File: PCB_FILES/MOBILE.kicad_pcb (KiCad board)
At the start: 2 copper layers, 88.6 x 52.6 mm, 33 parts, among them J1 Conn_01x05_Pin, Q1 MMBT3904_C181119, U1 HT7833, U2 ESP32-WROOM-32E-N8R2

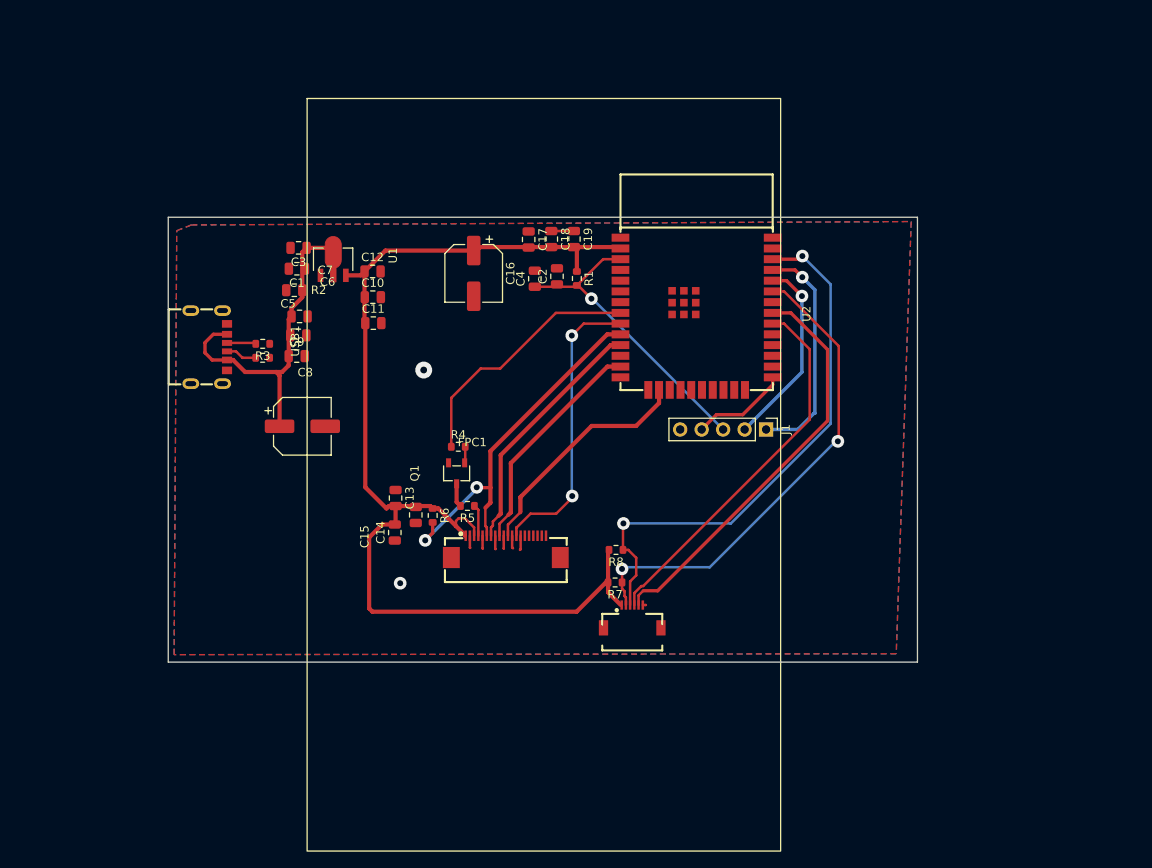
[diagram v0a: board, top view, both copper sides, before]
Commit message: 3rd commit
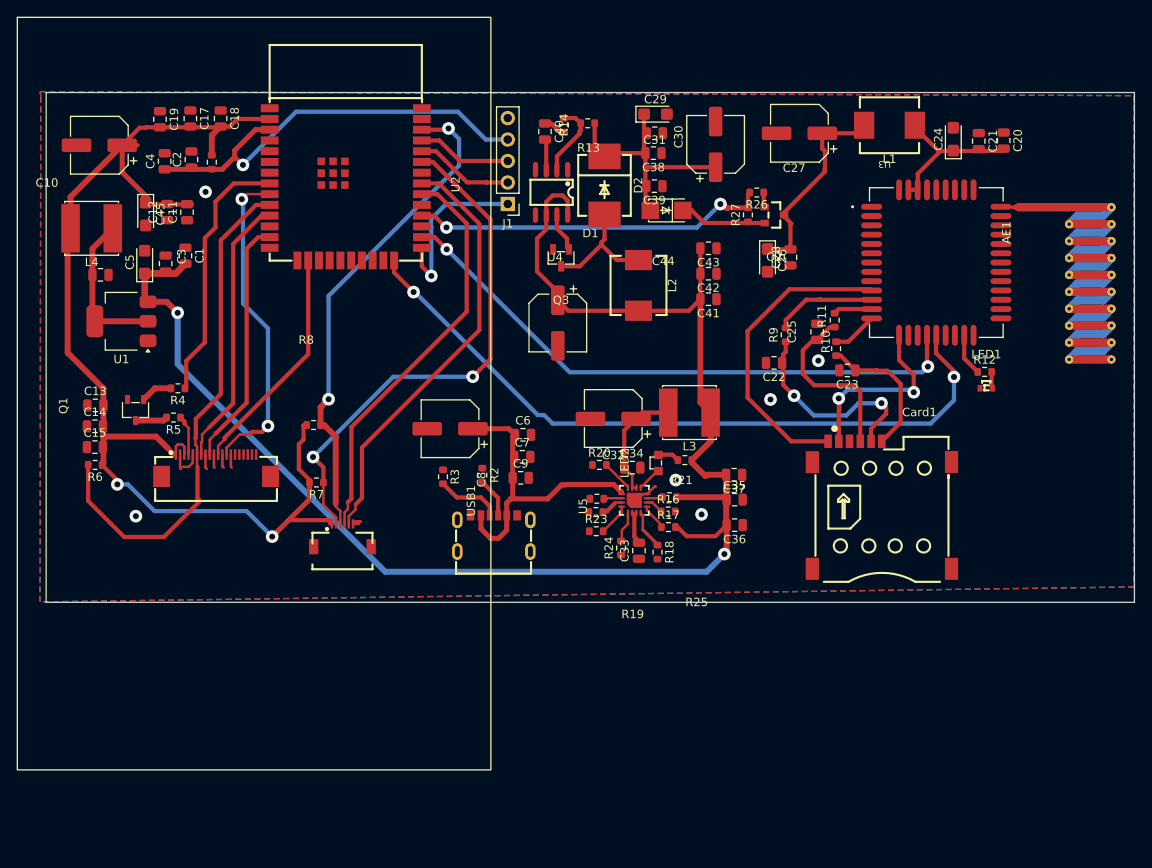
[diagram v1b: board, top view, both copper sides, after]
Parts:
- added AE1: Antenna, RF_Antenna:Texas_SWRA416_868MHz_915MHz, F.Cu at (159.2, 127.2)
- added C20: 100nF, Capacitor_SMD:C_0805_2012Metric, F.Cu at (152.3, 110.3)
- added C21: 33pF, Capacitor_SMD:C_0805_2012Metric, F.Cu at (149.3, 110.4)
- added C22: 33pF, Capacitor_SMD:C_0805_2012Metric, F.Cu at (125.1, 136.6)
- added C23: 33pF, Capacitor_SMD:C_0805_2012Metric, F.Cu at (133.8, 137.5)
- added C24: TAN 100uF, Capacitor_Tantalum_SMD:CP_EIA-3216-18_Kemet-A, F.Cu at (146.3, 110.2)
- added C25: 33pF, Capacitor_SMD:C_0805_2012Metric, F.Cu at (130.2, 133.0)
- added C26: TAN 100uF, Capacitor_Tantalum_SMD:CP_EIA-3216-18_Kemet-A, F.Cu at (124.4, 124.5)
- added C27: 470uF, Capacitor_SMD:CP_Elec_6.3x7.7, F.Cu at (128.1, 109.5)
- added C28: 22uF, Capacitor_SMD:C_0805_2012Metric, F.Cu at (127.1, 124.2)
- added C29: TAN 100uF, Capacitor_Tantalum_SMD:CP_EIA-3216-18_Kemet-A, F.Cu at (111.1, 107.2)
- added C30: 470uF, Capacitor_SMD:CP_Elec_6.3x7.7, F.Cu at (118.2, 110.8)
- added C31: 33pF, Capacitor_SMD:C_0805_2012Metric, F.Cu at (111.0, 109.5)
- added C32: 470uF, Capacitor_SMD:CP_Elec_6.3x7.7, F.Cu at (106.1, 143.2)
- added C33: 22uF, Capacitor_SMD:C_0805_2012Metric, F.Cu at (109.2, 158.8)
- added C34: 22uF, Capacitor_SMD:C_0805_2012Metric, F.Cu at (108.4, 149.0)
- added C35: 33pF, Capacitor_SMD:C_0805_2012Metric, F.Cu at (120.5, 152.8)
- added C36: 100nF, Capacitor_SMD:C_0805_2012Metric, F.Cu at (120.5, 155.8)
- added C37: 22uF, Capacitor_SMD:C_0805_2012Metric, F.Cu at (120.4, 149.9)
- added C38: 100nF, Capacitor_SMD:C_0805_2012Metric, F.Cu at (110.9, 111.8)
- added C39: 22uF, Capacitor_SMD:C_0805_2012Metric, F.Cu at (111.0, 115.7)
- added C40: 1uF, Capacitor_SMD:C_0805_2012Metric, F.Cu at (98.0, 109.3)
- added C41: 22uF, Capacitor_SMD:C_0805_2012Metric, F.Cu at (117.4, 129.1)
- added C42: 100nF, Capacitor_SMD:C_0805_2012Metric, F.Cu at (117.4, 126.1)
- added C43: 33pF, Capacitor_SMD:C_0805_2012Metric, F.Cu at (117.4, 123.1)
- added C44: 470uF, Capacitor_SMD:CP_Elec_6.3x7.7, F.Cu at (99.6, 131.9)
- added C45: TAN 10uF, Capacitor_Tantalum_SMD:CP_EIA-3216-18_Kemet-A, F.Cu at (50.8, 119.0)
- added Card1: SMC-202-6, easyeda2kicad:SIM-SMD_SMC-202-6, F.Cu at (137.9, 153.4)
- added D1: SS34, easyeda2kicad:DO-214AC_L4.3-W2.7-LS5.0-RD, F.Cu at (112.4, 118.6)
- added D2: B540C-13-F, easyeda2kicad:SMC_L7.1-W6.2-LS8.1-RD, F.Cu at (105.1, 115.6)
- added L1: MWSA0603S-4R7MT, easyeda2kicad:IND-SMD_L7.0-W6.6, F.Cu at (138.8, 108.5)
- added L2: MWSA0603S-4R7MT, easyeda2kicad:IND-SMD_L7.0-W6.6, F.Cu at (109.1, 127.5)
- added L3: CKCS6045-6.8UH/M, easyeda2kicad:IND-SMD_L6.0-W6.0, F.Cu at (115.1, 142.5)
- added L4: CKCS6045-6.8UH/M, easyeda2kicad:IND-SMD_L6.0-W6.0, F.Cu at (44.4, 120.7)
- added LED1: XL-1606UGC, easyeda2kicad:LED-SMD_L1.7-W1.1-R-RD_GREEN, F.Cu at (150.2, 139.6)
- added LED2: TZ-P2-0602RTS2-1.2T, easyeda2kicad:LED-SMD_L1.6-W1.2-RD, F.Cu at (111.5, 148.5)
- added Q2: SI2333, easyeda2kicad:SOT-23_L2.9-W1.3-P1.90-LS2.4-BR, F.Cu at (125.2, 119.1)
- added Q3: AP3404, easyeda2kicad:SOT-23-3_L2.9-W1.3-P1.90-LS2.4-BR-2, F.Cu at (100.0, 124.2)
- added R10: 22R, Resistor_SMD:R_0603_1608Metric, F.Cu at (132.5, 134.9)
- added R11: 22R, Resistor_SMD:R_0603_1608Metric, F.Cu at (132.3, 131.6)
- added R12: 1K, Resistor_SMD:R_0603_1608Metric, F.Cu at (150.0, 137.7)
- added R13: 68K, Resistor_SMD:R_0603_1608Metric, F.Cu at (103.1, 108.3)
- added R14: 27K, Resistor_SMD:R_0603_1608Metric, F.Cu at (100.3, 108.5)
- added R16: 100K, Resistor_SMD:R_0603_1608Metric, F.Cu at (112.6, 154.2)
- added R17: 10K, Resistor_SMD:R_0603_1608Metric, F.Cu at (112.7, 156.1)
- added R18: 10K, Resistor_SMD:R_0603_1608Metric, F.Cu at (111.4, 159.0)
- added R19: 51K, Resistor_SMD:R_0603_1608Metric, F.Cu at (104.2, 152.7)
- added R20: 1K1, Resistor_SMD:R_0603_1608Metric, F.Cu at (104.5, 148.7)
- added R21: 10K, Resistor_SMD:R_0603_1608Metric, F.Cu at (112.8, 152.5)
- added R22: 1K, Resistor_SMD:R_0603_1608Metric, F.Cu at (114.6, 148.1)
- added R23: 1K, Resistor_SMD:R_0603_1608Metric, F.Cu at (104.1, 156.5)
- added R24: 10K, Resistor_SMD:R_0603_1608Metric, F.Cu at (107.0, 158.5)
- added R25: 10K, Resistor_SMD:R_0603_1608Metric, F.Cu at (104.1, 154.3)
- added R26: 1K, Resistor_SMD:R_0603_1608Metric, F.Cu at (123.1, 116.5)
- added R27: 100K, Resistor_SMD:R_0603_1608Metric, F.Cu at (122.0, 119.1)
- added R9: 22R, Resistor_SMD:R_0603_1608Metric, F.Cu at (126.5, 133.3)
- added U3: M65, easyeda2kicad:XCVR_M65, F.Cu at (144.3, 124.8)
- added U4: ME2199ASG, easyeda2kicad:SOP-8_L4.9-W3.9-P1.27-LS6.0-BL, F.Cu at (98.8, 116.5)
- added U5: BQ24073RGTR, easyeda2kicad:QFN-16_L3.0-W3.0-P0.50-TL-EP1.7, F.Cu at (108.6, 152.9)
- C1: value 10uF -> 33pF
- C10: value 33pF -> 22uF
- C11: value 100nF -> 33pF
- C12: value 10uF -> 100nF
- C3: value 33pF -> 100nF
- C5: value 100nF -> TAN 10uF; footprint Capacitor_SMD:C_0805_2012Metric -> Capacitor_Tantalum_SMD:CP_EIA-3216-18_Kemet-A
- U1: value HT7833 -> AMS1117-3.3; footprint easyeda2kicad:SOT-89_L4.5-W2.5-P1.50-LS4.2-BR -> Package_TO_SOT_SMD:SOT-223-3_TabPin2
- moved C19 51.0 mm to (52.5, 107.8)
- moved C16 46.8 mm to (45.4, 110.9), turned to 180 degrees
- moved C4 45.9 mm to (53.1, 112.8)
- moved C2 45.4 mm to (56.2, 112.6)
- moved R1 45.3 mm to (58.6, 112.9)
- moved U2 44.2 mm to (74.5, 115.5)
- moved C17 42.5 mm to (56.1, 107.7)
- moved C18 41.6 mm to (59.7, 107.7)
- moved J1 40.6 mm to (93.7, 117.8), turned to 180 degrees
- moved R6 40.4 mm to (44.9, 148.7), turned to 180 degrees
- moved USB1 40.3 mm to (92.0, 156.8), turned to 0 degrees
- moved C15 38.8 mm to (44.8, 146.6), turned to 0 degrees
- moved Q1 38.7 mm to (49.6, 142.2)
- moved R8 38.7 mm to (70.7, 144.0)
- moved C14 37.6 mm to (44.8, 144.1), turned to 0 degrees
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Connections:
- C1 pad 1: +5V -> GND
- C1 pad 2: GND -> /VCC
- C10 pad 1: +3V3 -> GND
- C10 pad 2: GND -> Net-(U1-VO)
- C11 pad 1: +3V3 -> GND
- C11 pad 2: GND -> +3V3
- C12 pad 1: +3V3 -> GND
- C12 pad 2: GND -> +3V3
- C3 pad 1: +5V -> GND
- C3 pad 2: GND -> /VCC
- C5 pad 1: +5V -> /VCC
- J1 pad 1: /UOTXD -> /IO0
- J1 pad 3: /EN -> /UOTXD
- J1 pad 4: /IO0 -> /EN
- U1 pad 2: +5V -> Net-(U1-VO)
- U1 pad 3: +3V3 -> /VCC
- U2 pad 28: unconnected-(U2-IO17-Pad28) -> /IO17
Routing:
- net /VCC: track 0.00 -> 184.9 mm, vias 0 -> 2
- net /UART2_TX: track 0.00 -> 84.8 mm, vias 0 -> 2
- net /UART2_RX: track 0.00 -> 70.5 mm, vias 0 -> 2
- net /IO17: track 0.00 -> 42.4 mm, vias 0 -> 2
- net /SIM_GND: track 0.00 -> 36.3 mm
- net Net-(D1-A): track 0.00 -> 29.4 mm
- net /SIM_DATA: track 0.00 -> 24.4 mm, vias 0 -> 2
- net /VBAT: track 0.00 -> 24.3 mm
- net /SIM_VDD: track 0.00 -> 23.8 mm, vias 0 -> 2
- net /SIM_RST: track 0.00 -> 21.2 mm
- net /M65_PVR: track 0.00 -> 18.9 mm
- net Net-(U1-VO): track 0.00 -> 18.4 mm
- net /SIM_CLK: track 0.00 -> 16.7 mm
- net /LCD_CS: track 44.3 -> 60.7 mm, vias 2 -> 0
- net /EN: track 35.8 -> 51.9 mm
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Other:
- board size 88.6 x 52.6 mm -> 128.7 x 60.3 mm
